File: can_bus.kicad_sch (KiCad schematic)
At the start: 1 part, among them U8 MCP2562-E-SN

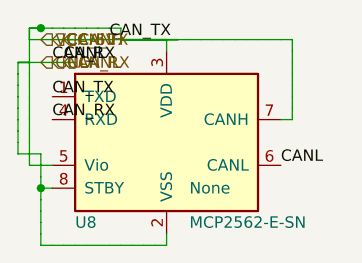
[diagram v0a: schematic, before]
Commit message: fix writer
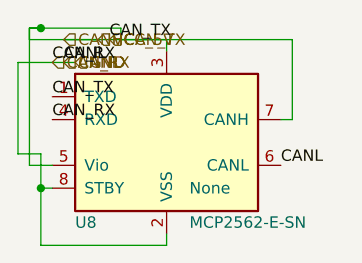
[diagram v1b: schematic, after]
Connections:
- net CANH: no longer U8.2 (VSS), U8.4 (RXD), U8.6 (CANL), U8.8 (STBY)
- new net CANL: U8.2 (VSS), U8.4 (RXD), U8.6 (CANL), U8.8 (STBY)
